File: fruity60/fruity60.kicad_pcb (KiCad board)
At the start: 2 copper layers, 132 parts

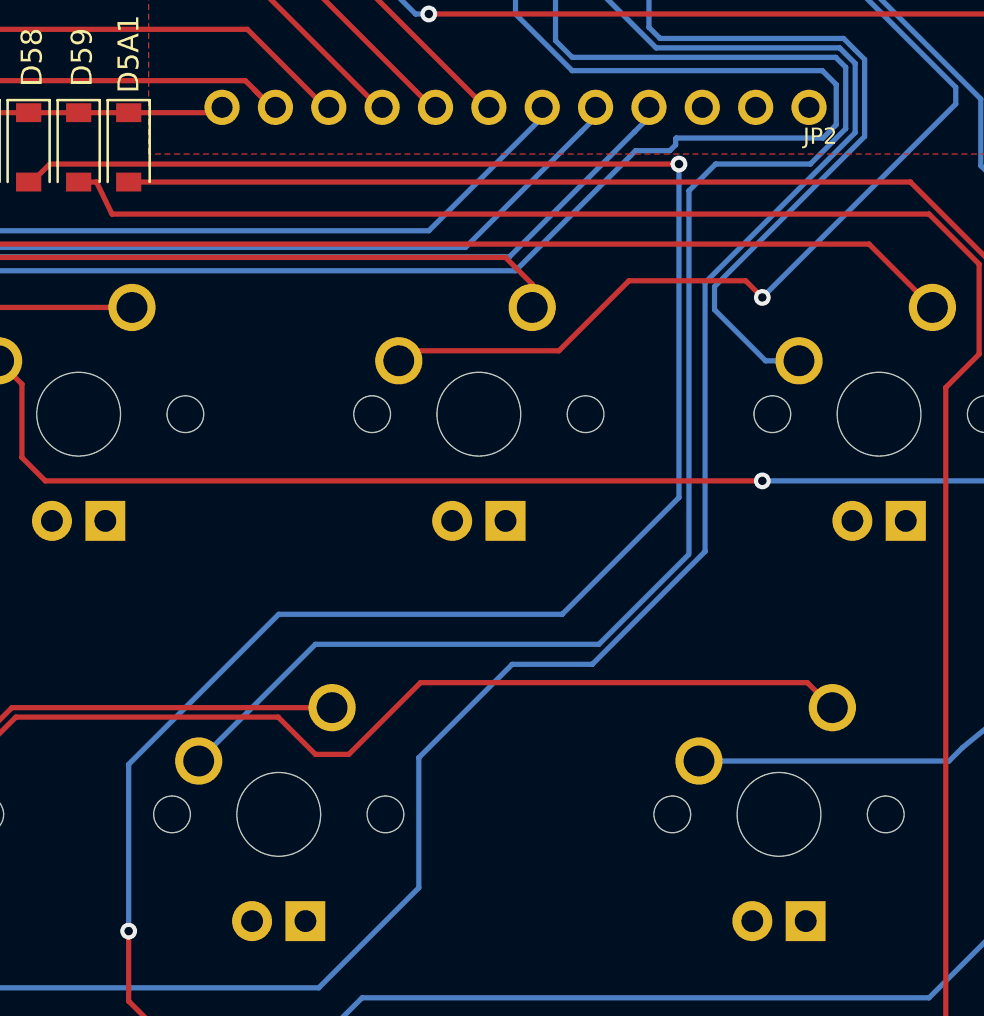
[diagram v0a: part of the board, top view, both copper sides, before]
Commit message: more clean ups
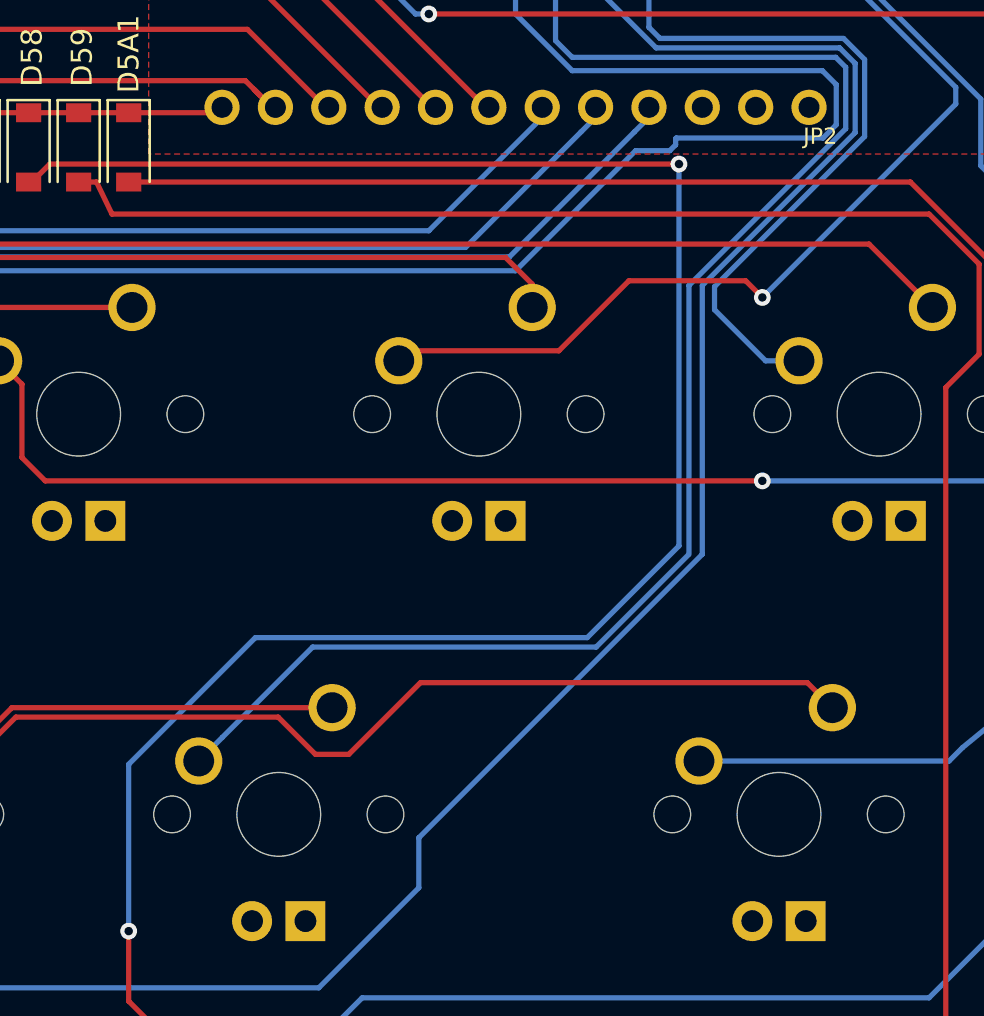
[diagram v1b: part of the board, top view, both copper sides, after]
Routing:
- net F0: track 552.5 -> 549.8 mm
- net F1: track 845.3 -> 843.0 mm
- net Net-(D58-Pad2): track 118.4 -> 119.7 mm
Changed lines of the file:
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@@
     (thickness 1.6)
     (drawings 42)
-    (tracks 1102)
+    (tracks 1099)
     (zones 0)
     (modules 132)
@@
   (segment (start 275.11375 64.77) (end 275.11375 64.77) (width 0.25) (layer F.Cu) (net 60))
   (via (at 275.11375 64.77) (size 0.8) (drill 0.4) (layers F.Cu B.Cu) (net 60))
-  (segment (start 275.11375 64.77) (end 275.11375 80.645) (width 0.25) (layer B.Cu) (net 60))
-  (segment (start 269.5575 86.20125) (end 256.06375 86.20125) (width 0.25) (layer B.Cu) (net 60))
-  (segment (start 275.11375 80.645) (end 269.5575 86.20125) (width 0.25) (layer B.Cu) (net 60))
-  (segment (start 256.06375 86.20125) (end 248.92 93.345) (width 0.25) (layer B.Cu) (net 60))
-  (segment (start 248.92 93.345) (end 248.92 101.2825) (width 0.25) (layer B.Cu) (net 60))
   (segment (start 248.92 101.2825) (end 248.92 101.2825) (width 0.25) (layer B.Cu) (net 60))
   (via (at 248.92 101.2825) (size 0.8) (drill 0.4) (layers F.Cu B.Cu) (net 60))
@@
   (segment (start 248.92 104.61625) (end 254 109.69625) (width 0.25) (layer F.Cu) (net 60))
   (segment (start 248.92 101.2825) (end 248.92 104.61625) (width 0.25) (layer F.Cu) (net 60))
+  (segment (start 254.9525 87.3125) (end 248.92 93.345) (width 0.25) (layer B.Cu) (net 60))
+  (segment (start 270.748125 87.3125) (end 254.9525 87.3125) (width 0.25) (layer B.Cu) (net 60))
+  (segment (start 248.92 93.345) (end 248.92 101.2825) (width 0.25) (layer B.Cu) (net 60))
+  (segment (start 275.11375 82.946875) (end 270.748125 87.3125) (width 0.25) (layer B.Cu) (net 60))
+  (segment (start 275.11375 64.77) (end 275.11375 82.946875) (width 0.25) (layer B.Cu) (net 60))
   (segment (start 262.57599 128.74625) (end 260.985 128.74625) (width 0.25) (layer F.Cu) (net 61))
   (segment (start 287.81375 109.274376) (end 267.602502 128.74625) (width 0.25) (layer F.Cu) (net 61))
@@
   (segment (start 103.66375 64.876269) (end 26.297198 64.876268) (width 0.25) (layer B.Cu) (net 64))
   (segment (start 109.37875 74.13625) (end 109.37875 70.591269) (width 0.25) (layer B.Cu) (net 64))
-  (segment (start 275.56376 83.36999) (end 271.30375 87.63) (width 0.25) (layer B.Cu) (net 64))
-  (segment (start 257.81 87.63) (end 252.25375 93.18625) (width 0.25) (layer B.Cu) (net 64))
-  (segment (start 271.30375 87.63) (end 257.81 87.63) (width 0.25) (layer B.Cu) (net 64))
   (segment (start 118.90375 92.86875) (end 118.90375 93.18625) (width 0.25) (layer B.Cu) (net 64))
   (segment (start 110.1725 84.1375) (end 118.90375 92.86875) (width 0.25) (layer B.Cu) (net 64))
@@
   (segment (start 268.605 41.75125) (end 268.605 42.936643) (width 0.25) (layer B.Cu) (net 64))
   (segment (start 269.24 43.571643) (end 269.24 47.625) (width 0.25) (layer B.Cu) (net 64))
-  (segment (start 276.86 64.77) (end 275.59 66.04) (width 0.25) (layer B.Cu) (net 64))
+  (segment (start 133.35 146.84375) (end 136.8425 150.33625) (width 0.25) (layer B.Cu) (net 64))
+  (segment (start 136.8425 150.33625) (end 147.47875 150.33625) (width 0.25) (layer B.Cu) (net 64))
+  (segment (start 133.35 131.445) (end 133.35 146.84375) (width 0.25) (layer B.Cu) (net 64))
+  (segment (start 133.19125 131.28625) (end 133.35 131.445) (width 0.25) (layer B.Cu) (net 64))
+  (segment (start 275.56376 83.36999) (end 271.171239 87.762511) (width 0.25) (layer B.Cu) (net 64))
+  (segment (start 271.171239 87.762511) (end 257.677489 87.762511) (width 0.25) (layer B.Cu) (net 64))
+  (segment (start 257.677489 87.762511) (end 253.378749 92.061251) (width 0.25) (layer B.Cu) (net 64))
+  (segment (start 253.378749 92.061251) (end 252.25375 93.18625) (width 0.25) (layer B.Cu) (net 64))
+  (segment (start 275.59 70.547502) (end 275.59 83.34375) (width 0.25) (layer B.Cu) (net 64))
+  (segment (start 283.05125 63.086252) (end 275.59 70.547502) (width 0.25) (layer B.Cu) (net 64))
   (segment (start 283.05125 60.16625) (end 283.05125 63.086252) (width 0.25) (layer B.Cu) (net 64))
   (segment (start 282.575 59.69) (end 283.05125 60.16625) (width 0.25) (layer B.Cu) (net 64))
   (segment (start 270.03375 59.69) (end 282.575 59.69) (width 0.25) (layer B.Cu) (net 64))
   (segment (start 269.24 58.89625) (end 270.03375 59.69) (width 0.25) (layer B.Cu) (net 64))
-  (segment (start 275.59 66.04) (end 275.59 83.34375) (width 0.25) (layer B.Cu) (net 64))
   (segment (start 269.24 47.663248) (end 269.24 58.89625) (width 0.25) (layer B.Cu) (net 64))
-  (segment (start 281.367502 64.77) (end 276.86 64.77) (width 0.25) (layer B.Cu) (net 64))
-  (segment (start 283.05125 63.086252) (end 281.367502 64.77) (width 0.25) (layer B.Cu) (net 64))
-  (segment (start 133.35 146.84375) (end 136.8425 150.33625) (width 0.25) (layer B.Cu) (net 64))
-  (segment (start 136.8425 150.33625) (end 147.47875 150.33625) (width 0.25) (layer B.Cu) (net 64))
-  (segment (start 133.35 131.445) (end 133.35 146.84375) (width 0.25) (layer B.Cu) (net 64))
-  (segment (start 133.19125 131.28625) (end 133.35 131.445) (width 0.25) (layer B.Cu) (net 64))
   (segment (start 270.306801 40.913051) (end 271.145 41.75125) (width 0.25) (layer B.Cu) (net 65))
   (segment (start 268.52497 39.13122) (end 270.306801 40.913051) (width 0.25) (layer B.Cu) (net 65))
@@
   (segment (start 91.28125 75.08875) (end 91.28125 84.61375) (width 0.25) (layer B.Cu) (net 65))
   (segment (start 90.32875 74.13625) (end 91.28125 75.08875) (width 0.25) (layer B.Cu) (net 65))
+  (segment (start 113.016251 130.161251) (end 114.14125 131.28625) (width 0.25) (layer B.Cu) (net 65))
+  (segment (start 105.56875 122.71375) (end 113.016251 130.161251) (width 0.25) (layer B.Cu) (net 65))
+  (segment (start 105.56875 113.18875) (end 105.56875 122.71375) (width 0.25) (layer B.Cu) (net 65))
+  (segment (start 104.61625 112.23625) (end 105.56875 113.18875) (width 0.25) (layer B.Cu) (net 65))
   (segment (start 234.15625 95.72974) (end 233.20375 94.77724) (width 0.25) (layer B.Cu) (net 65))
   (segment (start 234.15625 103.1875) (end 234.15625 95.72974) (width 0.25) (layer B.Cu) (net 65))
   (segment (start 234.95 103.98125) (end 234.15625 103.1875) (width 0.25) (layer B.Cu) (net 65))
+  (segment (start 257.96875 103.98125) (end 234.95 103.98125) (width 0.25) (layer B.Cu) (net 65))
+  (segment (start 233.20375 94.77724) (end 233.20375 93.18625) (width 0.25) (layer B.Cu) (net 65))
+  (segment (start 271.145 56.35766) (end 274.027329 59.239989) (width 0.25) (layer B.Cu) (net 65))
   (segment (start 262.73125 99.21875) (end 257.96875 103.98125) (width 0.25) (layer B.Cu) (net 65))
   (segment (start 271.145 41.75125) (end 271.145 56.35766) (width 0.25) (layer B.Cu) (net 65))
-  (segment (start 262.73125 93.0275) (end 262.73125 99.21875) (width 0.25) (layer B.Cu) (net 65))
-  (segment (start 267.17625 88.5825) (end 262.73125 93.0275) (width 0.25) (layer B.Cu) (net 65))
-  (segment (start 270.98766 88.5825) (end 267.17625 88.5825) (width 0.25) (layer B.Cu) (net 65))
-  (segment (start 276.35751 70.416402) (end 276.35751 83.21265) (width 0.25) (layer B.Cu) (net 65))
-  (segment (start 276.35751 83.21265) (end 270.98766 88.5825) (width 0.25) (layer B.Cu) (net 65))
-  (segment (start 283.501261 63.272652) (end 276.35751 70.416402) (width 0.25) (layer B.Cu) (net 65))
-  (segment (start 283.501261 59.97985) (end 283.501261 63.272652) (width 0.25) (layer B.Cu) (net 65))
-  (segment (start 233.20375 94.77724) (end 233.20375 93.18625) (width 0.25) (layer B.Cu) (net 65))
+  (segment (start 262.73125 96.83891) (end 262.73125 99.21875) (width 0.25) (layer B.Cu) (net 65))
+  (segment (start 276.225 83.34516) (end 262.73125 96.83891) (width 0.25) (layer B.Cu) (net 65))
+  (segment (start 276.225 70.548913) (end 276.225 83.34516) (width 0.25) (layer B.Cu) (net 65))
+  (segment (start 283.501261 63.272652) (end 276.225 70.548913) (width 0.25) (layer B.Cu) (net 65))
   (segment (start 282.7614 59.239989) (end 283.501261 59.97985) (width 0.25) (layer B.Cu) (net 65))
+  (segment (start 283.501261 59.97985) (end 283.501261 63.272652) (width 0.25) (layer B.Cu) (net 65))
   (segment (start 274.027329 59.239989) (end 282.7614 59.239989) (width 0.25) (layer B.Cu) (net 65))
-  (segment (start 257.96875 103.98125) (end 234.95 103.98125) (width 0.25) (layer B.Cu) (net 65))
-  (segment (start 271.145 56.35766) (end 274.027329 59.239989) (width 0.25) (layer B.Cu) (net 65))
-  (segment (start 113.016251 130.161251) (end 114.14125 131.28625) (width 0.25) (layer B.Cu) (net 65))
-  (segment (start 105.56875 122.71375) (end 113.016251 130.161251) (width 0.25) (layer B.Cu) (net 65))
-  (segment (start 105.56875 113.18875) (end 105.56875 122.71375) (width 0.25) (layer B.Cu) (net 65))
-  (segment (start 104.61625 112.23625) (end 105.56875 113.18875) (width 0.25) (layer B.Cu) (net 65))
   (segment (start 272.846801 40.913051) (end 273.685 41.75125) (width 0.25) (layer B.Cu) (net 66))
   (segment (start 270.61496 38.68121) (end 272.846801 40.913051) (width 0.25) (layer B.Cu) (net 66))
